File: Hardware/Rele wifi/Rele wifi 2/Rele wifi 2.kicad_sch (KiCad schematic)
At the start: 9 parts, among them J1 Screw_Terminal_01x02, J2 Screw_Terminal_01x03, K1 G5LE-1, Q1 BC337, U1 PC817, U3 ESP8266-DEVKITC-02U-F

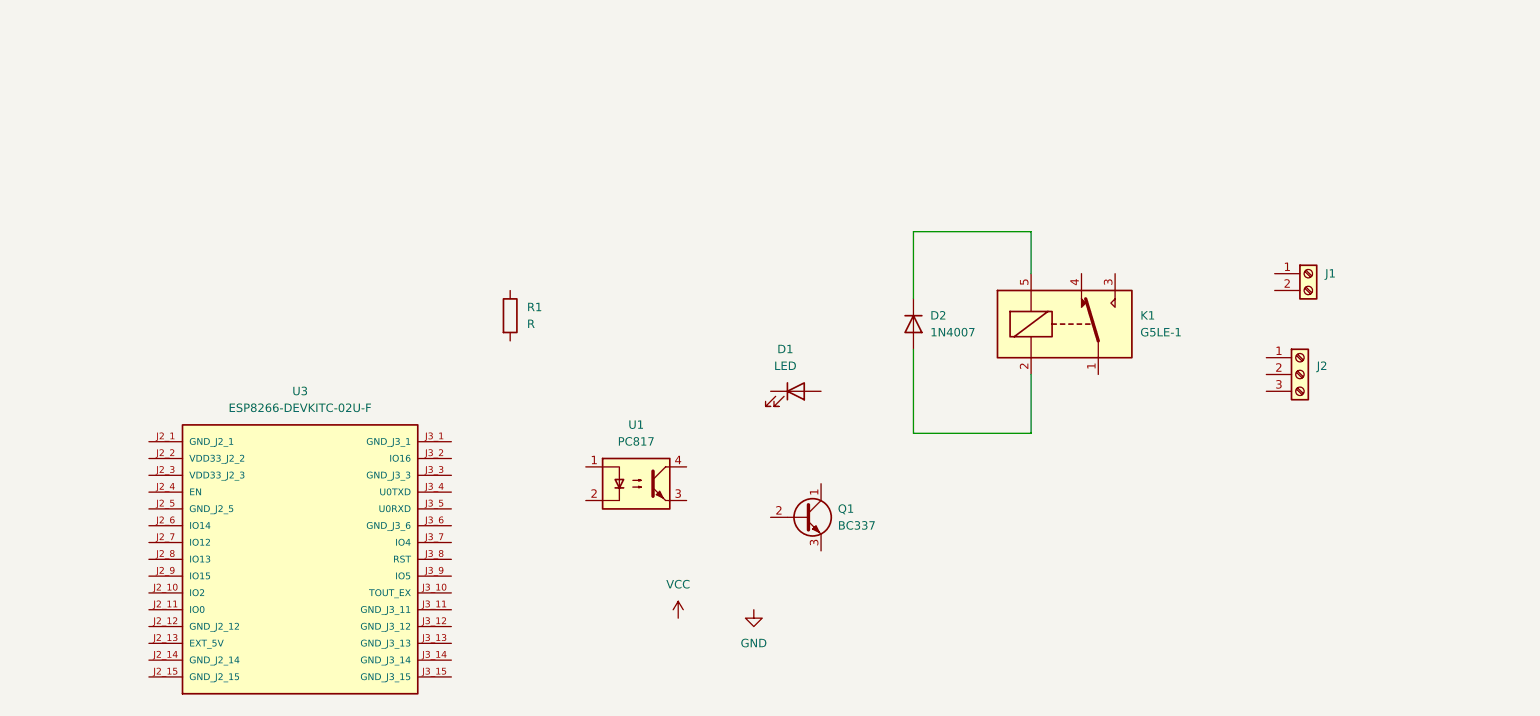
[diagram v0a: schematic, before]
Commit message: rele 2
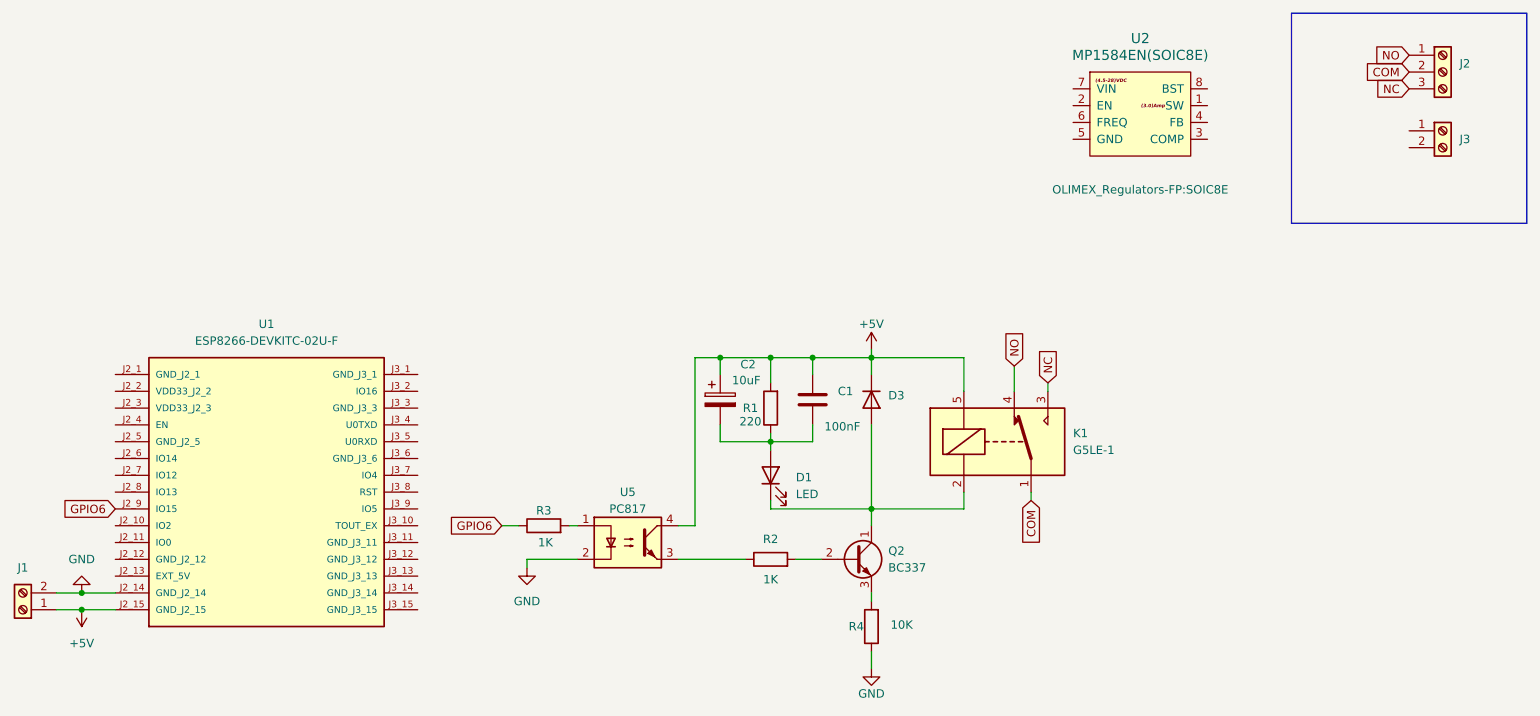
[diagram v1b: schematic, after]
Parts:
- removed D2: 1N4007, Diode_THT:D_DO-41_SOD81_P10.16mm_Horizontal, symbol Diode:1N4007
- removed Q1: BC337, Package_TO_SOT_THT:TO-92_Inline, symbol Transistor_BJT:BC337
- removed U1: PC817, Package_DIP:DIP-4_W7.62mm, symbol Isolator:PC817
- removed U3: ESP8266-DEVKITC-02U-F, ESP8266-DEVKITC-02U-F:MODULE_ESP8266-DEVKITC-02U-F, symbol ESP8266-DEVKITC-02U-F:ESP8266-DEVKITC-02U-F
- added C1: 100nF, Capacitor_THT:C_Disc_D4.7mm_W2.5mm_P5.00mm, symbol Device:C
- added C2: 10uF, Capacitor_THT:CP_Radial_D5.0mm_P2.00mm, symbol Device:C_Polarized
- added D3: 1N4007, Diode_THT:D_DO-41_SOD81_P12.70mm_Horizontal, symbol local_lib:1N4007
- added J3: Screw_Terminal_01x02, TerminalBlock:TerminalBlock_MaiXu_MX126-5.0-02P_1x02_P5.00mm, symbol Connector:Screw_Terminal_01x02
- added Q2: BC337, Package_TO_SOT_THT:TO-92_Inline, symbol Transistor_BJT:BC337
- added R2, R3: 1K, Resistor_SMD:R_0805_2012Metric, symbol Device:R
- added R4: 10K, Resistor_SMD:R_0805_2012Metric, symbol Device:R
- added U1: ESP8266-DEVKITC-02U-F, ESP8266:ESP12F-Devkit-V3, symbol ESP8266-DEVKITC-02U-F:ESP8266-DEVKITC-02U-F
- added U2: MP1584EN(SOIC8E), OLIMEX_Regulators-FP:SOIC8E, symbol OLIMEX_Regulators:MP1584EN(SOIC8E)
- added U5: PC817, Package_SO:SOP-4_7.5x4.1mm_P2.54mm, symbol local_lib:PC817
- D1: footprint (none) -> LED_THT:LED_D3.0mm_Clear
- J1: footprint (none) -> TerminalBlock:TerminalBlock_MaiXu_MX126-5.0-02P_1x02_P5.00mm
- J2: footprint (none) -> TerminalBlock:TerminalBlock_MaiXu_MX126-5.0-03P_1x03_P5.00mm
- R1: value R -> 220; footprint (none) -> Resistor_SMD:R_0805_2012Metric
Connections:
- net GND: now also J1.2 (Pin_2), R4.1, U1.J2_14 (GND_J2_14), U5.2
- net at R1.1: now also D1.2 (A), C1.2, C2.2
- net +5V: now reaches R1.2
- net +5V: now also J1.1 (Pin_1), K1.5, C1.1, C2.1, D3.1 (K), U1.J2_15 (GND_J2_15), U5.4
- net at D1.1 (K): now also K1.2, D3.2 (A), Q2.1 (C)
- net NO: now reaches J2.1 (Pin_1)
- net NO: now also K1.4
- net COM: now reaches J2.2 (Pin_2)
- net COM: now also K1.1
- net NC: now reaches J2.3 (Pin_3)
- net NC: now also K1.3
- new net: R3.2, U5.1
- new net: R2.1, U5.3
- new net: Q2.3 (E), R4.2
- new net: Q2.2 (B), R2.2
- new net: U2.5 (GND), U2.EP1
- new net GPIO6: R3.1, U1.J2_9 (IO15)
